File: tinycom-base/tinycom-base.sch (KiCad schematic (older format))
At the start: 9 parts, among them J1 MICRO_SD_HINGE, P1 CONN_02X08, P2 CONN_02X08, P3 USB_A, P4 CONN_01X12, P5 CONN_02X12, U1 OLIMEX_IC_AXP209, U2 STM32-48PIN, U3 fpc_24

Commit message: add base
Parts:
- removed P4: CONN_01X12, Pin_Headers:Pin_Header_Straight_1x12, symbol CONN_01X12
- removed P5: CONN_02X12, Pin_Headers:Pin_Header_Straight_2x12, symbol CONN_02X12
- removed U2: STM32-48PIN, mods:QFP50P900X900X160-48N, symbol STM32-48PIN
- removed U3: fpc_24, tinycom:fpc_24, symbol fpc_24
- added P4: USB_B, Connect:USB_Micro-B, symbol USB_B
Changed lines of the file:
@@
 LIBS:armory
 LIBS:stm32-48pin-devBoard
-LIBS:tinycom-pwm-cache
 EELAYER 25 0
 EELAYER END
@@
 $EndComp
 $Comp
-L CONN_02X12 P5
-U 1 1 562C6235
-P 4950 6400
-F 0 "P5" H 4950 7050 50  0000 C CNN
-F 1 "CONN_02X12" V 4950 6400 50  0000 C CNN
-F 2 "Pin_Headers:Pin_Header_Straight_2x12" H 4950 5200 60  0001 C CNN
-F 3 "" H 4950 5200 60  0000 C CNN
-	1    4950 6400
+L USB_B P4
+U 1 1 562CE6C3
+P 5200 6000
+F 0 "P4" H 5400 5800 50  0000 C CNN
+F 1 "USB_B" H 5150 6200 50  0000 C CNN
+F 2 "Connect:USB_Micro-B" V 5150 5900 60  0001 C CNN
+F 3 "" V 5150 5900 60  0000 C CNN
+	1    5200 6000
 	1    0    0    -1
 $EndComp
-$Comp
-L CONN_01X12 P4
-U 1 1 562C6348
-P 4450 6400
-F 0 "P4" H 4450 7050 50  0000 C CNN
-F 1 "CONN_01X12" V 4550 6400 50  0000 C CNN
-F 2 "Pin_Headers:Pin_Header_Straight_1x12" H 4450 6400 60  0001 C CNN
-F 3 "" H 4450 6400 60  0000 C CNN
-	1    4450 6400
-	1    0    0    -1
-$EndComp
-$Comp
-L STM32-48PIN U2
-U 1 1 562C67D9
-P 9350 2650
-F 0 "U2" H 8350 4400 60  0000 C CNN
-F 1 "STM32-48PIN" H 8600 850 60  0000 C CNN
-F 2 "mods:QFP50P900X900X160-48N" H 9350 2650 60  0001 C CNN
-F 3 "" H 9350 2650 60  0000 C CNN
-	1    9350 2650
-	1    0    0    -1
-$EndComp
-$Comp
-L fpc_24 U3
-U 1 1 562CDBDB
-P 9250 5050
-F 0 "U3" H 9250 5050 60  0000 C CNN
-F 1 "fpc_24" H 9250 5050 60  0000 C CNN
-F 2 "tinycom:fpc_24" H 9250 5050 60  0000 C CNN
-F 3 "" H 9250 5050 60  0000 C CNN
-	1    9250 5050
-	1    0    0    -1
-$EndComp

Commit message: xxx
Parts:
- U1: footprint ax209:ax209-OLIMEX_IC_QFN48 -> tinycom:ax209-OLIMEX_IC_QFN48
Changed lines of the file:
@@
 F 0 "U1" H 2350 6280 50  0000 L BNN
 F 1 "OLIMEX_IC_AXP209" H 2350 1250 50  0000 L BNN
-F 2 "ax209:ax209-OLIMEX_IC_QFN48" H 2850 4000 50  0001 C CNN
+F 2 "tinycom:ax209-OLIMEX_IC_QFN48" H 2850 4000 50  0001 C CNN
 F 3 "" H 2850 3850 60  0000 C CNN
 	1    2850 3850

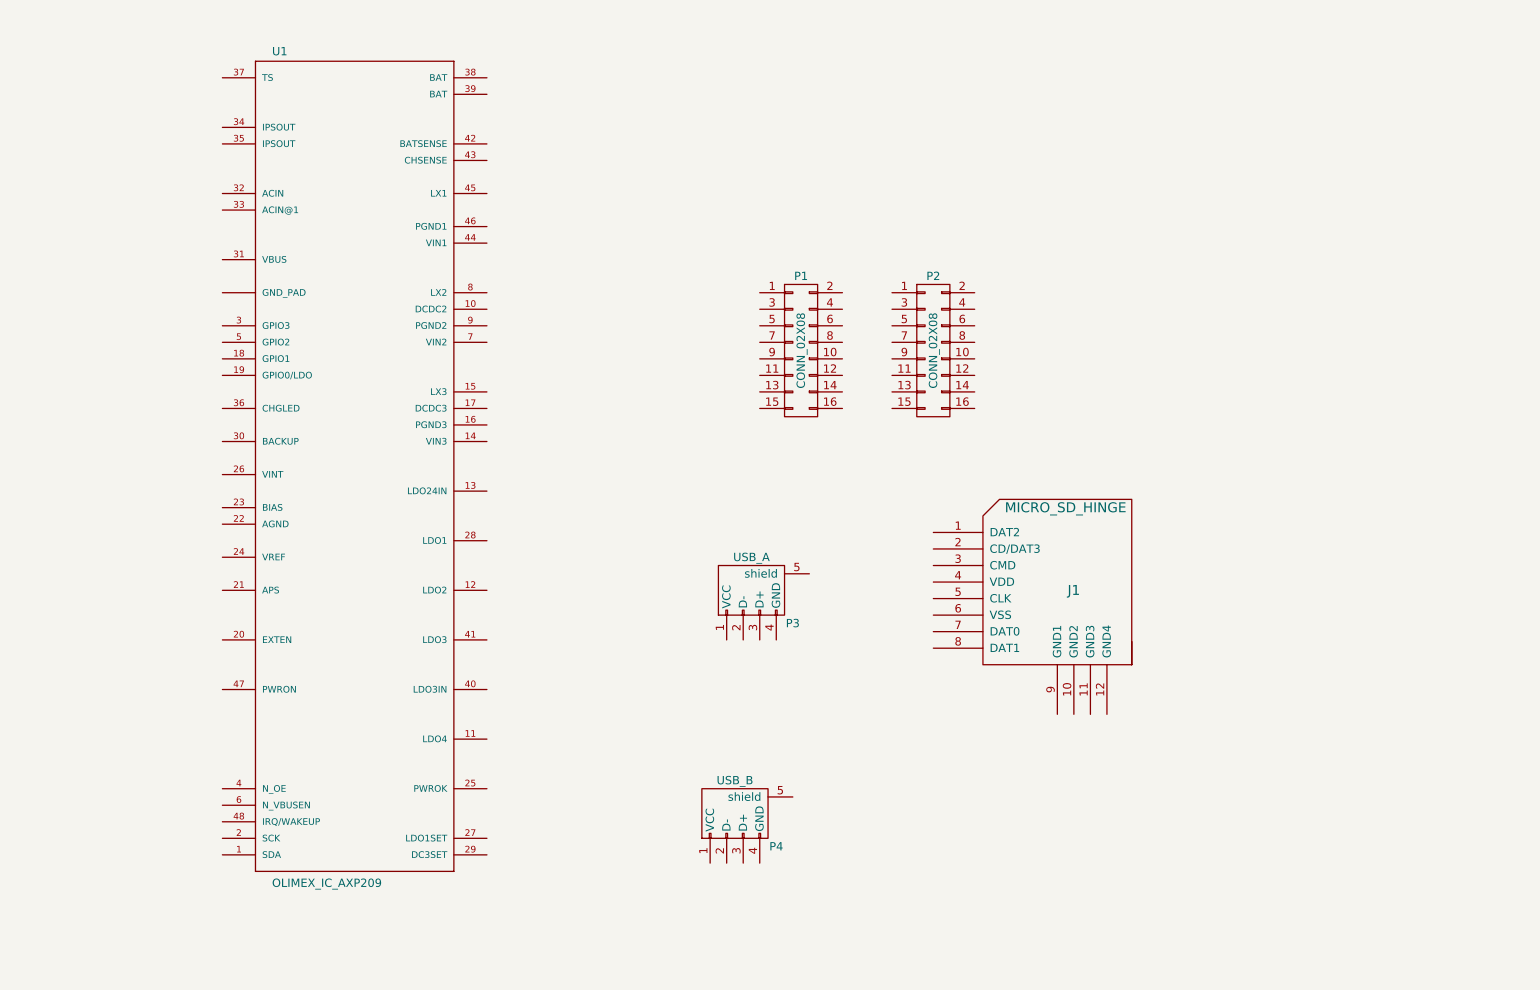
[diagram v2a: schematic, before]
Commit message: prepare base
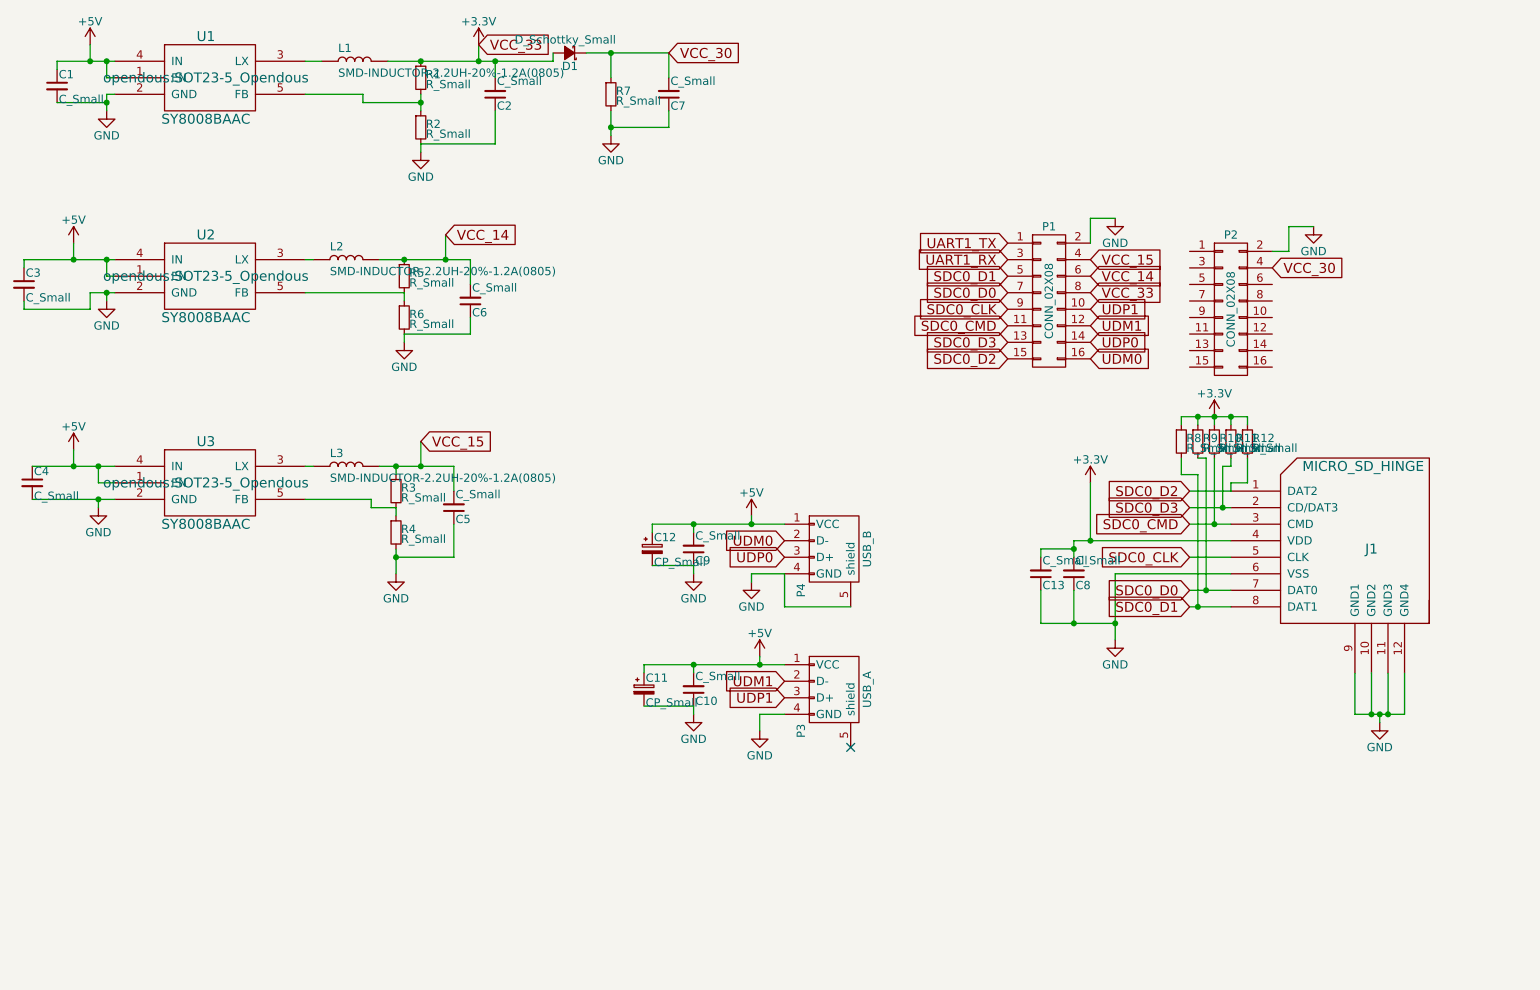
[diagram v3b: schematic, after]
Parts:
- removed U1: OLIMEX_IC_AXP209, tinycom:ax209-OLIMEX_IC_QFN48, symbol OLIMEX_IC_AXP209
- added C1, C10, C13, C2, C3, C4, C5, C6, C7, C8, C9: C_Small, Capacitors_SMD:C_0805, symbol C_Small
- added C11, C12: CP_Small, Capacitors_Elko_ThroughHole:Elko_vert_11.2x6.3mm_RM2.5_CopperClear, symbol CP_Small
- added D1: D_Schottky_Small, Diodes_SMD:SMA_Standard, symbol D_Schottky_Small
- added L1, L2, L3: SMD-INDUCTOR-2.2UH-20%-1.2A(0805), cd32:CD32, symbol SMD-INDUCTOR-2.2UH-20%-1.2A(0805)
- added R1, R10, R11, R12, R2, R3, R4, R5, R6, R7, R8, R9: R_Small, Resistors_SMD:R_0805, symbol R_Small
- added U1, U2, U3: SY8008BAAC, opendous:SOT23-5_Opendous, symbol SY8008BAAC
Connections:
- net UART1_TX: now reaches P1.1 (P1)
- net UDP1: now reaches P1.10 (P10)
- net UDP1: now also P3.3 (D+)
- net SDC0_CMD: now reaches P1.11 (P11)
- net SDC0_CMD: now also J1.3 (CMD), R10.2
- net UDM1: now reaches P1.12 (P12)
- net UDM1: now also P3.2 (D-)
- net SDC0_D3: now reaches P1.13 (P13)
- net SDC0_D3: now also J1.2 (CD/DAT3), R11.2
- net UDP0: now reaches P1.14 (P14)
- net UDP0: now also P4.3 (D+)
- net SDC0_D2: now reaches P1.15 (P15)
- net SDC0_D2: now also J1.1 (DAT2), R12.2
- net UDM0: now reaches P1.16 (P16)
- net UDM0: now also P4.2 (D-)
- net GND: now reaches P1.2 (P2)
- net GND: now also J1.10 (GND2), J1.11 (GND3), J1.12 (GND4), J1.6 (VSS), J1.9 (GND1), P2.2 (P2), P3.4 (GND), P4.4 (GND), P4.5 (shield), C1.2, C10.1, C11.2, C12.2, C13.1, C2.1, C3.2, C4.2, C5.1, C6.1, C7.1, C8.1, C9.1, R2.2, R4.2, R6.2, R7.2, U1.2 (GND), U2.2 (GND), U3.2 (GND)
- net UART1_RX: now reaches P1.3 (P3)
- net VCC_15: now reaches P1.4 (P4)
- net VCC_15: now also C5.2, L3.2, R3.1
- net SDC0_D1: now reaches P1.5 (P5)
- net SDC0_D1: now also J1.8 (DAT1), R8.2
- net VCC_14: now reaches P1.6 (P6)
- net VCC_14: now also C6.2, L2.2, R5.1
- net SDC0_D0: now reaches P1.7 (P7)
- net SDC0_D0: now also J1.7 (DAT0), R9.2
- net +3V3: now reaches P1.8 (P8)
- net +3V3: now also J1.4 (VDD), C13.2, C2.2, C8.2, D1.2 (A), L1.2, R1.1, R10.1, R11.1, R12.1, R8.1, R9.1
- net SDC0_CLK: now reaches P1.9 (P9)
- net SDC0_CLK: now also J1.5 (CLK)
- net VCC_30: now reaches P2.4 (P4)
- net VCC_30: now also C7.2, D1.1 (K), R7.1
- net +5V: now reaches P3.1 (VCC)
- net +5V: now also P4.1 (VCC), C1.1, C10.2, C11.1, C12.1, C3.1, C4.1, C9.2, U1.1 (EN), U1.4 (IN), U2.1 (EN), U2.4 (IN), U3.1 (EN), U3.4 (IN)
- new net: L1.1, U1.3 (LX)
- new net: R1.2, R2.1, U1.5 (FB)
- new net: L2.1, U2.3 (LX)
- new net: R5.2, R6.1, U2.5 (FB)
- new net: L3.1, U3.3 (LX)
- new net: R3.2, R4.1, U3.5 (FB)
- no-connect marks 0 -> 1
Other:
- moved on the sheet: J1, P1, P2, P3, P4
